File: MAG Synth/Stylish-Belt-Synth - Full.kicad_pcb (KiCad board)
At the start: 2 copper layers, 177.8 x 101.7 mm, 67 parts, among them J0 USB_B, J1 Audio-Jack-3_2Switches, J26 WRITE PATCH, J27 PARAM SELECT, J28 PATCH SELECT, J29 MODE, J30 STYLUS, SW1 Power, U1 stm32f103c8t6-module-china, U2 XPT8871

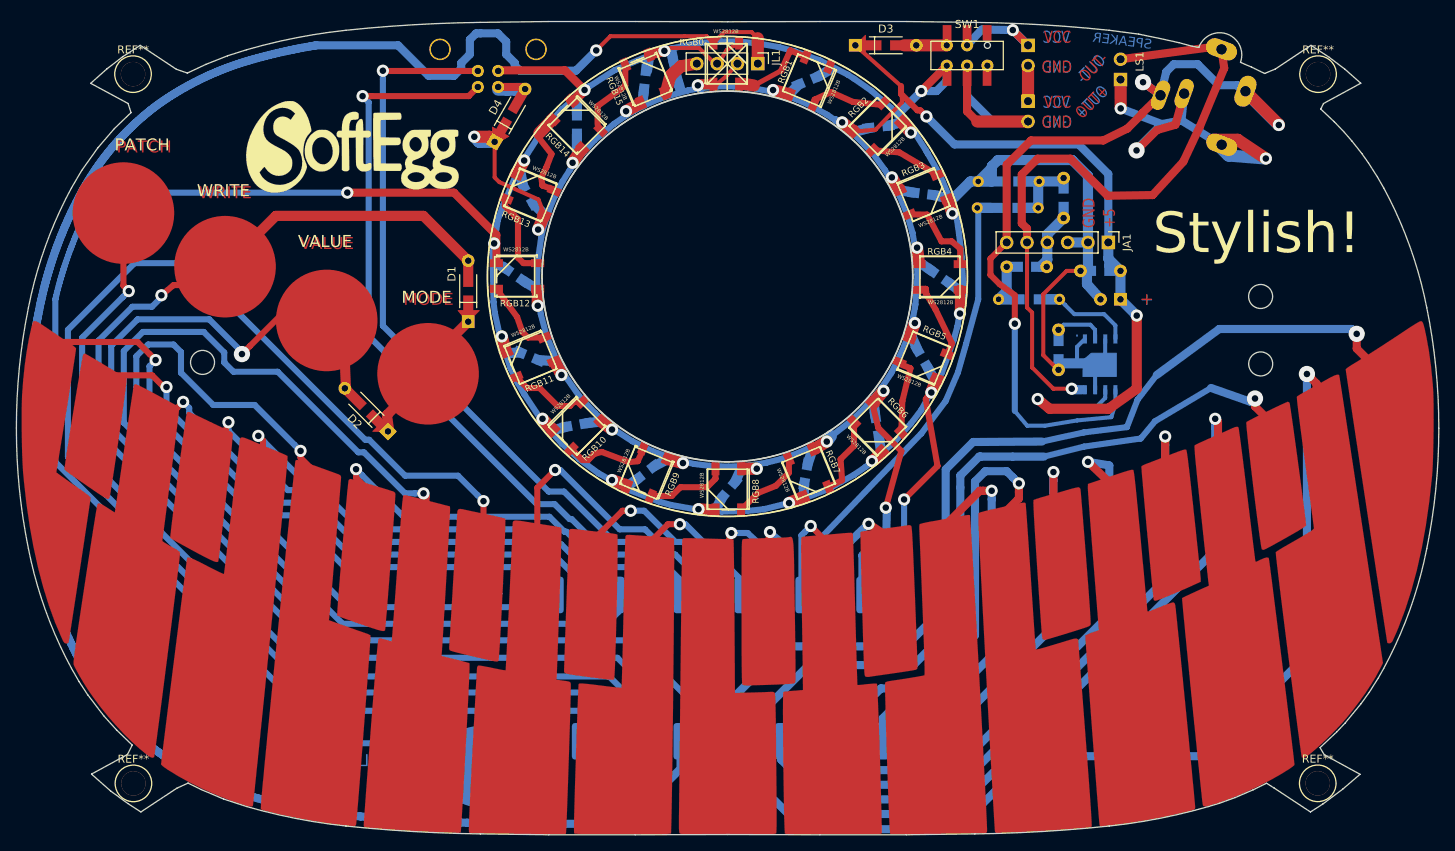
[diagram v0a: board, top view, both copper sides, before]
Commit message: V3 board V2.4 case
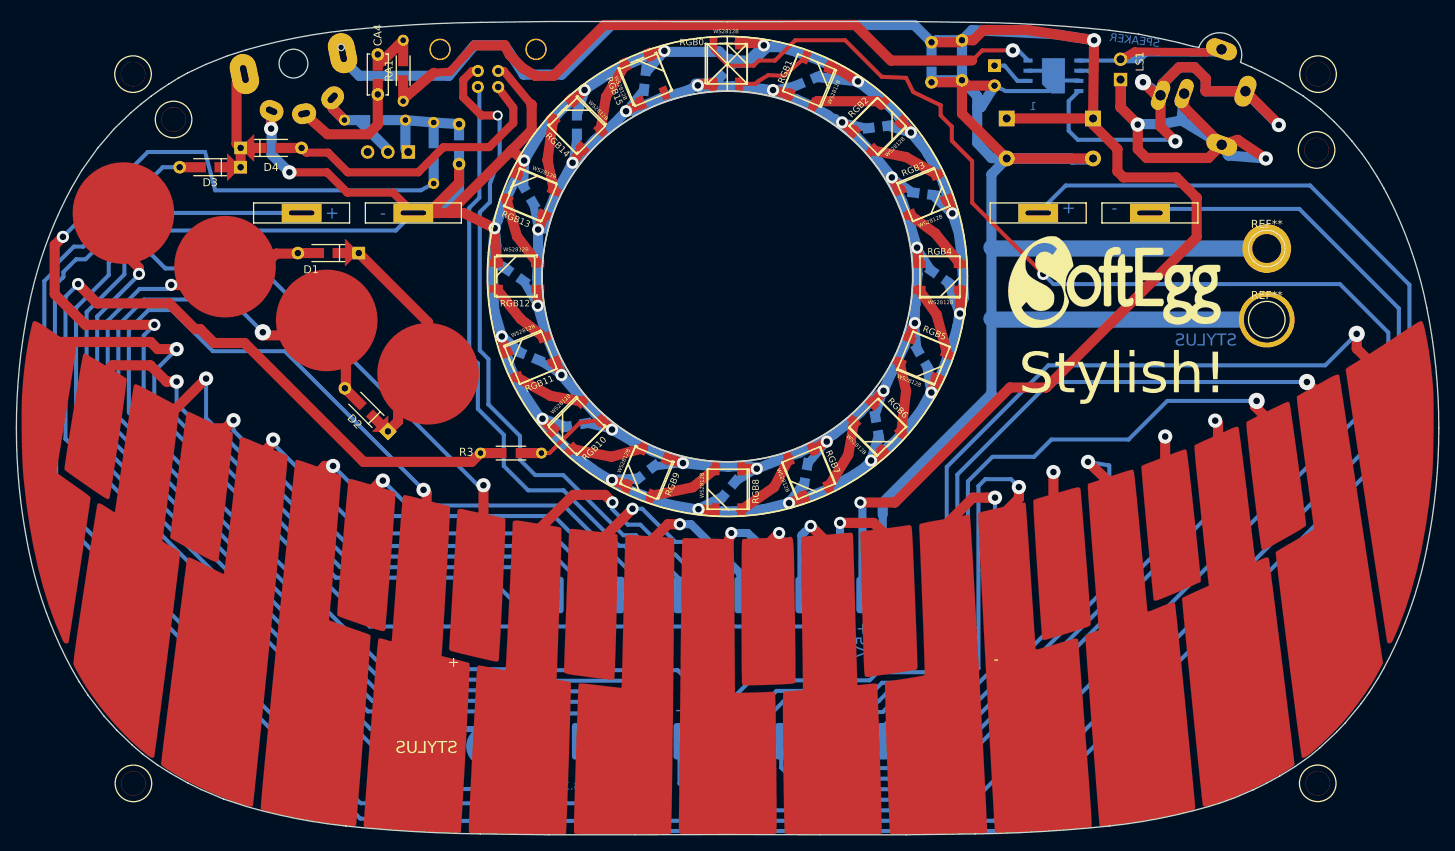
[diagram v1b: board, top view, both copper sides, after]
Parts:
- removed BT1: 4 x 1.5V, Pin_Headers:Pin_Header_Straight_1x02_Pitch2.54mm
- removed BT2: Conn_01x02, Pin_Headers:Pin_Header_Straight_1x02_Pitch2.54mm
- removed JA1: Conn_01x06, Pin_Headers:Pin_Header_Straight_1x06_Pitch2.54mm
- removed JL1: ~, Pin_Headers:Pin_Header_Straight_1x04_Pitch2.54mm
- removed the REF** at (215.1, 104.8)
- removed the REF** at (82.9, 104.6)
- added ?: 1pin, Connect:1pin, F.Cu at (79.2, 66.4)
- added ?: 1pin, Connect:1pin, F.Cu at (222.1, 70.2)
- added BT12: ~, SoftEggKiCAD:AA_Battery_Dual_Terminal, B.Cu at (95.2, 134.2)
- added BT34: ~, SoftEggKiCAD:AA_Battery_Dual_Terminal, B.Cu at (187.3, 134.0)
- added BTN1: -, SoftEggKiCAD:AA_Battery_-_Terminal, B.Cu at (109.2, 78.1)
- added BTN3: -, SoftEggKiCAD:AA_Battery_-_Terminal, B.Cu at (201.3, 78.1)
- added BTP2: +, SoftEggKiCAD:AA_Battery_+_Terminal, B.Cu at (95.2, 78.1)
- added BTP4: +, SoftEggKiCAD:AA_Battery_+_Terminal, B.Cu at (187.3, 78.1)
- added C2: 1000μF, Capacitors_ThroughHole:CP_Radial_D10.0mm_P5.00mm, B.Cu at (194.2, 66.3)
- added C3: 470μF, Capacitors_ThroughHole:CP_Radial_D10.0mm_P5.00mm, B.Cu at (183.4, 66.3)
- added RA1: 100Ω, SoftEggKiCAD:R_Axial_DIN0204_L3.6mm_D1.6mm_P7.62mm_Horizontal+SMD804, F.Cu at (108.0, 64.1)
- added REF**: 1pin, Connectors:1pin, F.Cu at (215.9, 82.5)
- added REF**: 1pin, Connectors:1pin, F.Cu at (215.9, 91.4)
- added RV1: Volume, SoftEggKiCAD:Wheel_Pot_W_Switch_RV12_B103_FUSTAR, B.Cu at (94.2, 59.4)
- CA1: footprint Capacitors_ThroughHole:CP_Radial_Tantal_D4.5mm_P2.50mm -> SoftEggKiCAD:C_Disc_D5.0mm_W2.5mm_P5.00mm+SMD
- CA3: footprint SoftEggKiCAD:C_Disc_D5.0mm_W2.5mm_P5.00mm+SMD -> Capacitors_ThroughHole:CP_Radial_Tantal_D4.5mm_P2.50mm
- CA4: moved to F.Cu
- J1: value Audio-Jack-3_2Switches -> Headphone
- LS1: value SPEAKER -> Speaker
- R1: value 10kΩ -> 8Ω
- R2: value 1k -> 47Ω
- R3: value 100Ω -> 120Ω; moved to F.Cu
- SW1: value Power -> OVERDRIVE; footprint SoftEggKiCAD:MSS22D18+THT -> Pin_Headers:Pin_Header_Straight_1x03_Pitch2.54mm; moved to B.Cu
- moved G*** 96.7 mm to (196.8, 86.7)
- moved CA4 83.0 mm to (104.8, 58.3), turned to 270 degrees
- moved R2 79.6 mm to (100.6, 66.5)
- moved D3 78.3 mm to (87.6, 72.4), turned to 180 degrees
- moved C1 76.5 mm to (114.9, 67.0), turned to 270 degrees
- moved R1 76.3 mm to (111.8, 66.8), turned to 270 degrees
- moved SW1 70.9 mm to (108.6, 70.5), turned to 90 degrees
- moved R3 67.6 mm to (125.2, 108.1)
- moved CA1 39.9 mm to (174.0, 56.8), turned to 270 degrees
- moved U2 36.5 mm to (189.2, 61.0), turned to 90 degrees
- moved CA2 35.0 mm to (177.8, 56.5), turned to 270 degrees
- moved CA3 34.0 mm to (181.9, 59.7)
- moved D4 31.8 mm to (87.6, 70.0), turned to 0 degrees
- moved D1 16.1 mm to (102.4, 83.1), turned to 180 degrees
- moved CL0 6.46 mm to (148.5, 60.2), turned to 45 degrees
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- renumbered REF** to ?
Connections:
- C1 pad 1: /PWM_OUT -> Net-(C1-Pad1)
- C1 pad 2: Net-(C1-Pad2) -> GND
- CL0 pad 1: /+5V -> /VIN
- CL1 pad 1: /+5V -> /VIN
- CL10 pad 1: /+5V -> /VIN
- CL11 pad 1: /+5V -> /VIN
- CL12 pad 1: /+5V -> /VIN
- CL13 pad 1: /+5V -> /VIN
- CL14 pad 1: /+5V -> /VIN
- CL15 pad 1: /+5V -> /VIN
- CL2 pad 1: /+5V -> /VIN
- CL3 pad 1: /+5V -> /VIN
- CL4 pad 1: /+5V -> /VIN
- CL5 pad 1: /+5V -> /VIN
- CL6 pad 1: /+5V -> /VIN
- CL7 pad 1: /+5V -> /VIN
- CL8 pad 1: /+5V -> /VIN
- CL9 pad 1: /+5V -> /VIN
- D3 pad 1: /+5V -> /VUSB
- D3 pad 2: Net-(D3-Pad2) -> Net-(BTP4-Pad1)
- D4 pad 1: /+5V -> /VUSB
- J1 pad 1: /XH-M125-amp-board/OUT+ -> Net-(J1-Pad1)
- J1 pad 2: /XH-M125-amp-board/OUT+ -> Net-(J1-Pad1)
- J1 pad 3: /XH-M125-amp-board/OUT- -> Net-(J1-Pad3)
- LS1 pad 2: /XH-M125-amp-board/OUT- -> Net-(J1-Pad3)
- R1 pad 1: Net-(C1-Pad2) -> Net-(C1-Pad1)
- R2 pad 1: GND -> Net-(R2-Pad1)
- R2 pad 2: Net-(C1-Pad2) -> Net-(C1-Pad1)
- R3 pad 1: Net-(R3-Pad1) -> /VIN
- R3 pad 2: Net-(CA4-Pad1) -> /+3.3V
- RGB0 pad 1: /+5V -> /VIN
- RGB1 pad 1: /+5V -> /VIN
- RGB10 pad 1: /+5V -> /VIN
- RGB11 pad 1: /+5V -> /VIN
- RGB12 pad 1: /+5V -> /VIN
- RGB13 pad 1: /+5V -> /VIN
- RGB14 pad 1: /+5V -> /VIN
- RGB15 pad 1: /+5V -> /VIN
- RGB15 pad 2: /WS2812B-16-LED-RING/DOUT -> /DOUT
- RGB2 pad 1: /+5V -> /VIN
- RGB3 pad 1: /+5V -> /VIN
- RGB4 pad 1: /+5V -> /VIN
- RGB5 pad 1: /+5V -> /VIN
- RGB6 pad 1: /+5V -> /VIN
- RGB7 pad 1: /+5V -> /VIN
- RGB8 pad 1: /+5V -> /VIN
- RGB9 pad 1: /+5V -> /VIN
- U1 pad 38: Net-(U1-Pad38) -> /+3.3V
- U2 pad 4: Net-(R3-Pad1) -> Net-(RA1-Pad1)
- U2 pad 5: /XH-M125-amp-board/OUT+ -> Net-(J1-Pad3)
- U2 pad 8: /XH-M125-amp-board/OUT- -> Net-(J1-Pad1)
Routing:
- net Net-(BTP4-Pad1): track 0.00 -> 330.3 mm
- net Net-(BTN3-Pad1): track 0.00 -> 317.1 mm
- net /VIN: track 0.00 -> 248.2 mm, vias 0 -> 16
- net GND: track 549.0 -> 728.0 mm, vias 17 -> 18
- net /+3.3V: track 0.00 -> 166.0 mm, vias 0 -> 1
- net /AUDIO_OUT: track 58.4 -> 183.9 mm, vias 0 -> 2
- net /+5V: track 364.2 -> 244.8 mm, vias 21 -> 2
- net /XH-M125-amp-board/OUT+: track 104.1 -> 0.00 mm, vias 3 -> 0
- net Net-(RA1-Pad1): track 0.00 -> 90.2 mm, vias 0 -> 1
- net /XH-M125-amp-board/OUT-: track 84.7 -> 0.00 mm, vias 1 -> 0
- net Net-(J1-Pad1): track 0.00 -> 77.0 mm, vias 0 -> 3
- net /F0: track 111.6 -> 47.4 mm
- net Net-(J1-Pad3): track 0.00 -> 31.1 mm
- net Net-(D4-Pad2): track 6.87 -> 35.3 mm
- net /WRITE: track 151.2 -> 123.9 mm
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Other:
- outline, holes or cut-outs redrawn
- net class Default: trace_width 0.2 -> 0.635; via_dia 2.032 -> 1.524
- board text added: "+5V"
- board text added: "-"
- board text added: "3.3V"
- board text added: "AUD"
- board text added: "L"
- board text removed: "+5"
- board text removed: "."
- board text removed: "MODE"
- board text removed: "OUT+"
- board text removed: "OUT-"
- board text removed: "PATCH"
- board text removed: "VALUE"
- board text removed: "VCC"
- board text removed: "WRITE"
